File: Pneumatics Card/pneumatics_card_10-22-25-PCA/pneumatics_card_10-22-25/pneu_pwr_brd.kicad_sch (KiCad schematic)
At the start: 57 parts, among them J2 2X1, J3 2X1, J4 2X1, J5 2X1, J6 2X1, J7 2X1, Q3 FQP30N06L, Q4 FQP30N06L, Q5 FQP30N06L, Q6 FQP30N06L, Q7 IRF4905SPbF, U1 L7805, U2 LD1117V33, U3 PCA9685, U4 MCP1416, U5 TCA4307, U6 MCP1416, U7 MCP1416, U8 MCP1416

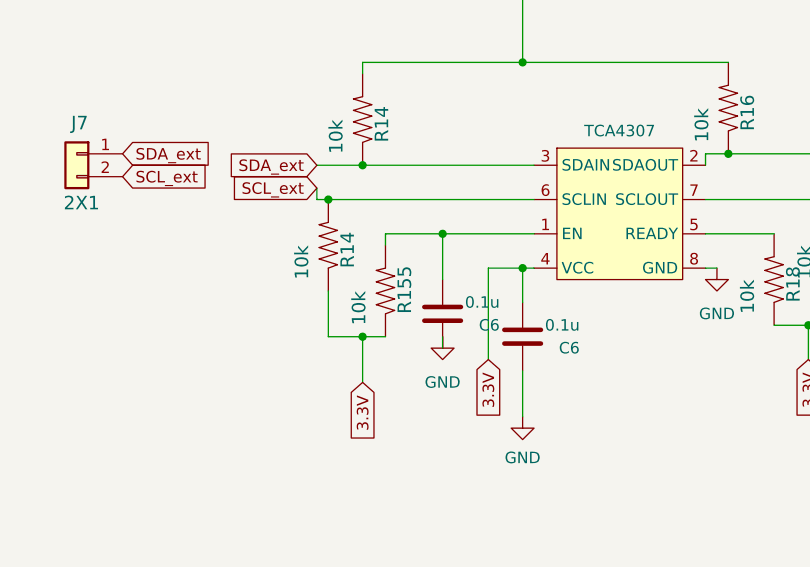
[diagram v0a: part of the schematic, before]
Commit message: testing
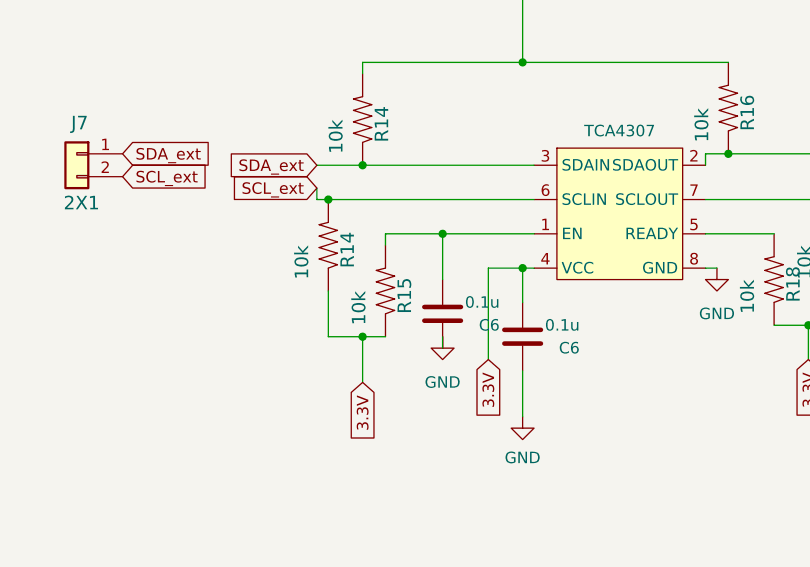
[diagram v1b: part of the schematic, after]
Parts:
- renumbered R155 to R15
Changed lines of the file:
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@@
 		(on_board yes)
 		(dnp no)
-		(property "Reference" "R155"
+		(property "Reference" "R15"
 			(at 68.58 49.53 0)
 			(effects
@@
 			(project "pneu_pwr_brd"
 				(path "/c299c6f2-212e-472c-8577-e7ed124513dd"
-					(reference "R155")
+					(reference "R15")
 					(unit 1)
 				)
